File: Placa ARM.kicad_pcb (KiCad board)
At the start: 2 copper layers, 69.5 x 31.9 mm, 39 parts, among them J1 USB_B_Micro, J2 Conn_ARM_JTAG_SWD_10, J3 Conn_01x12, J4 Conn_01x12, J5 Conn_02x04_Odd_Even, SW1 SW_Push_Dual, U1 XR21B1411IL16TR-F, U2 SP6260GEK-L_TR, U3 LMV358AIDR, U4 EFM32TG11B120F128GM32, Y1 32MHz, Y2 32.768KHz

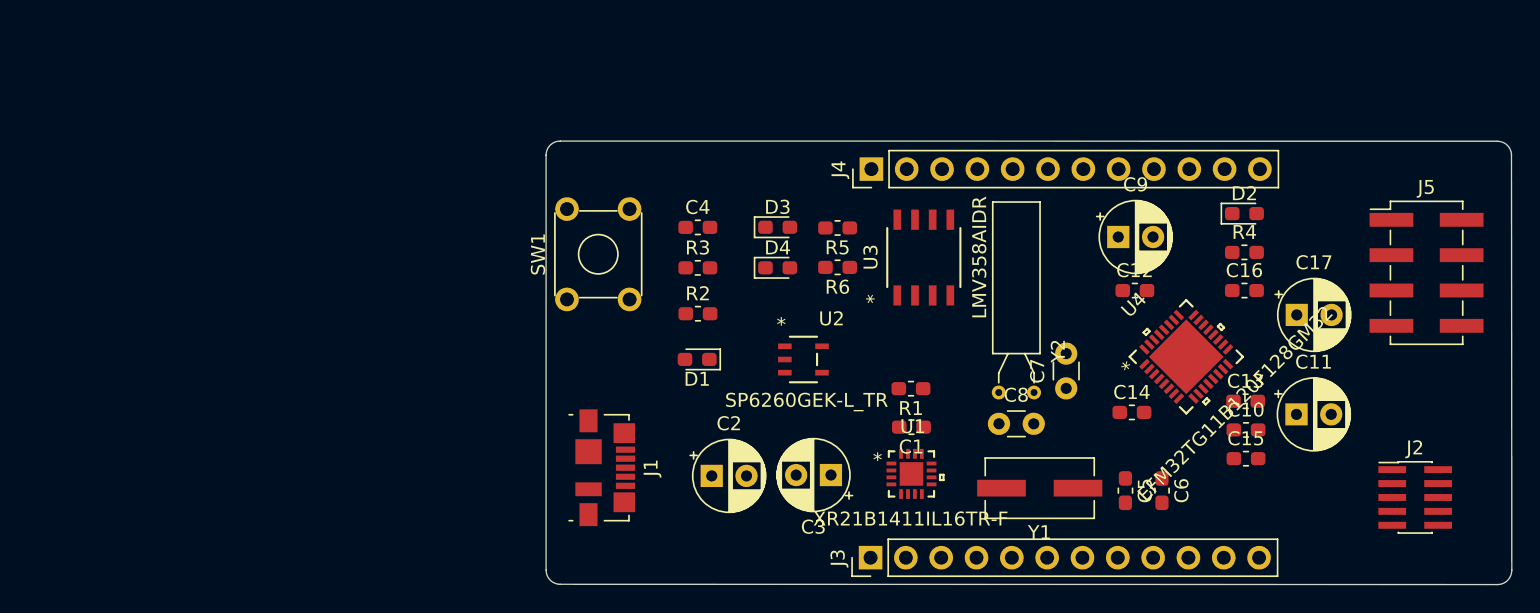
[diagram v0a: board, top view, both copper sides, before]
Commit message: Issue #2: PCB lista para primera prueba de concepto
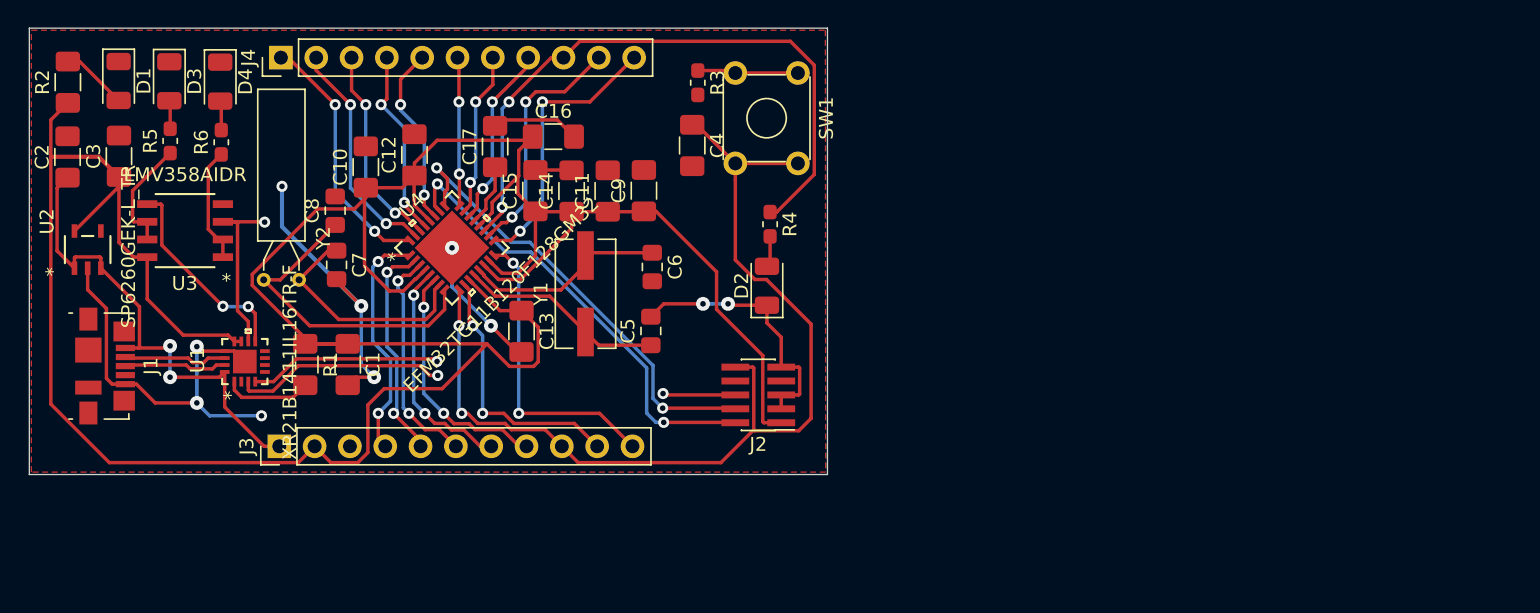
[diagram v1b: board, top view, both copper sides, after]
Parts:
- removed J5: Conn_02x04_Odd_Even, Connector_PinHeader_2.54mm:PinHeader_2x04_P2.54mm_Vertical_SMD
- C1, C10, C12, C13, C14, C15, C16, C4: footprint Capacitor_SMD:C_0603_1608Metric_Pad1.05x0.95mm_HandSolder -> Capacitor_SMD:C_1206_3216Metric_Pad1.42x1.75mm_HandSolder
- C11, C17, C2, C3, C9: footprint Capacitor_THT:CP_Radial_D5.0mm_P2.50mm -> Capacitor_SMD:C_1206_3216Metric_Pad1.42x1.75mm_HandSolder
- C5, C6: footprint Capacitor_SMD:C_0603_1608Metric_Pad1.05x0.95mm_HandSolder -> Capacitor_SMD:C_0805_2012Metric_Pad1.15x1.40mm_HandSolder
- C7, C8: footprint Capacitor_THT:C_Disc_D3.0mm_W1.6mm_P2.50mm -> Capacitor_SMD:C_0805_2012Metric_Pad1.15x1.40mm_HandSolder
- D1, D2, D3, D4: footprint LED_SMD:LED_0603_1608Metric_Pad1.05x0.95mm_HandSolder -> LED_SMD:LED_1206_3216Metric
- J3, J4: value Conn_01x12 -> Conn_01x11; footprint Connector_PinHeader_2.54mm:PinHeader_1x12_P2.54mm_Vertical -> Connector_PinHeader_2.54mm:PinHeader_1x11_P2.54mm_Vertical
- R1, R2: footprint Resistor_SMD:R_0603_1608Metric_Pad1.05x0.95mm_HandSolder -> Resistor_SMD:R_1206_3216Metric_Pad1.42x1.75mm_HandSolder
- moved C10 66.1 mm to (71.6, 103.8), turned to 90 degrees
- moved C17 58.9 mm to (80.9, 102.3), turned to 90 degrees
- moved C3 56.1 mm to (53.9, 103.0), turned to 90 degrees
- moved C15 54.6 mm to (83.8, 105.5), turned to 90 degrees
- moved Y2 53.5 mm to (66.8, 111.9)
- moved U4 53.4 mm to (77.8, 109.6)
- moved C7 53.2 mm to (69.5, 110.8), turned to 270 degrees
- moved U3 53.2 mm to (58.6, 108.4), turned to 180 degrees
- moved C12 52.7 mm to (75.1, 102.9), turned to 90 degrees
- moved C13 52.3 mm to (82.8, 115.6), turned to 270 degrees
- moved U2 52.1 mm to (51.6, 109.7), turned to 90 degrees
- moved C11 52.1 mm to (89.0, 105.5), turned to 90 degrees
- moved C2 51.7 mm to (50.1, 103.1), turned to 90 degrees
- moved C16 50.9 mm to (85.1, 101.6)
- moved C8 50.1 mm to (69.4, 106.9), turned to 90 degrees
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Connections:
- J1 pad 6: GND -> Net-(J1-Pad6)
- J3 pad 1: /IU5 -> +5V
- J3 pad 10: /Interfaz de Usuario/MCU_PE11 -> /Interfaz de Usuario/MCU_PB11
- J3 pad 11: /Interfaz de Usuario/MCU_PE12 -> /Interfaz de Usuario/MCU_PD4
- J3 pad 3: +5V -> GND
- J3 pad 4: GND -> /Interfaz de Usuario/MCU_PA0
- J3 pad 5: /Interfaz de Usuario/MCU_PA0 -> /Interfaz de Usuario/MCU_PA1
- J3 pad 6: /Interfaz de Usuario/MCU_PA1 -> /Interfaz de Usuario/MCU_PA2
- J3 pad 7: /Interfaz de Usuario/MCU_PA2 -> /Interfaz de Usuario/MCU_PC0
- J3 pad 8: /Interfaz de Usuario/MCU_PB11 -> /Interfaz de Usuario/MCU_PC1
- J3 pad 9: /Interfaz de Usuario/MCU_PE10 -> /IU5
- J4 pad 1: /Interfaz de Usuario/MCU_PF0 -> /Interfaz de Usuario/MCU_PE13
- J4 pad 10: /IU8 -> /IU9
- J4 pad 11: /IU9 -> /IU8
- J4 pad 2: /IU6 -> /Interfaz de Usuario/MCU_PE12
- J4 pad 3: /IU7 -> /Interfaz de Usuario/MCU_PE11
- J4 pad 4: /Interfaz de Usuario/MCU_PC0 -> /Interfaz de Usuario/MCU_PE10
- J4 pad 5: /Interfaz de Usuario/MCU_PC1 -> /IU7
- J4 pad 6: /Interfaz de Usuario/MCU_PC13 -> /Interfaz de Usuario/MCU_PC15
- J4 pad 8: /Interfaz de Usuario/MCU_PC15 -> /Interfaz de Usuario/MCU_PC13
- J4 pad 9: /Interfaz de Usuario/MCU_PD4 -> /Interfaz de Usuario/MCU_PD7
- U1 pad 5: /IU1 -> Net-(U1-Pad5)
- U1 pad 6: /IU2 -> Net-(U1-Pad6)
- U1 pad 7: /IU3 -> Net-(U1-Pad7)
- U1 pad 8: /IU4 -> Net-(U1-Pad8)
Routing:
- net +3V3: track 0.00 -> 223.8 mm
- net GND: track 0.00 -> 87.9 mm, vias 0 -> 10
- net /IU5: track 0.00 -> 72.6 mm, vias 0 -> 2
- net /Interfaz de Usuario/MCU_PD7: track 0.00 -> 46.7 mm, vias 0 -> 2
- net /IU6: track 0.00 -> 45.6 mm, vias 0 -> 3
- net +5V: track 0.00 -> 34.9 mm, vias 0 -> 2
- net /IU8: track 0.00 -> 33.9 mm, vias 0 -> 3
- net /Interfaz de Usuario/MCU_PF0: track 0.00 -> 33.3 mm, vias 0 -> 2
- net /IU7: track 0.00 -> 33.0 mm, vias 0 -> 5
- net /IU9: track 0.00 -> 32.8 mm, vias 0 -> 3
- net /Microcontrolador/MCU_PB8: track 0.00 -> 23.1 mm
- net /Interfaz de Usuario/MCU_PD4: track 0.00 -> 21.8 mm, vias 0 -> 2
- net /Interfaz de Usuario/MCU_PB11: track 0.00 -> 19.0 mm, vias 0 -> 2
- net /Interfaz de Usuario/MCU_PE13: track 0.00 -> 18.4 mm, vias 0 -> 2
- net /Interfaz de Usuario/MCU_PC1: track 0.00 -> 17.5 mm, vias 0 -> 2
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- added copper zone on F.Cu, net GND
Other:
- board size 69.5 x 31.9 mm -> 57.4 x 32.1 mm
- net class Power added: clearance 0.2, trace_width 0.3, via_dia 1, via_drill 0.4
